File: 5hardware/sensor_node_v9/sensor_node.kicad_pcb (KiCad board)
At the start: 2 copper layers, 11.6 x 19.6 mm, 24 parts, among them J1 Conn_01x04_Pin, J3 Conn_01x04_Pin, Q1 BC818, Q2 Si2371EDS, Q3 AO3400A, U12 APDS-9960, U13 SHT31-DIS, U17 BH1750FVI-TR, U7 XC6206PxxxMR, U8 TPL5110

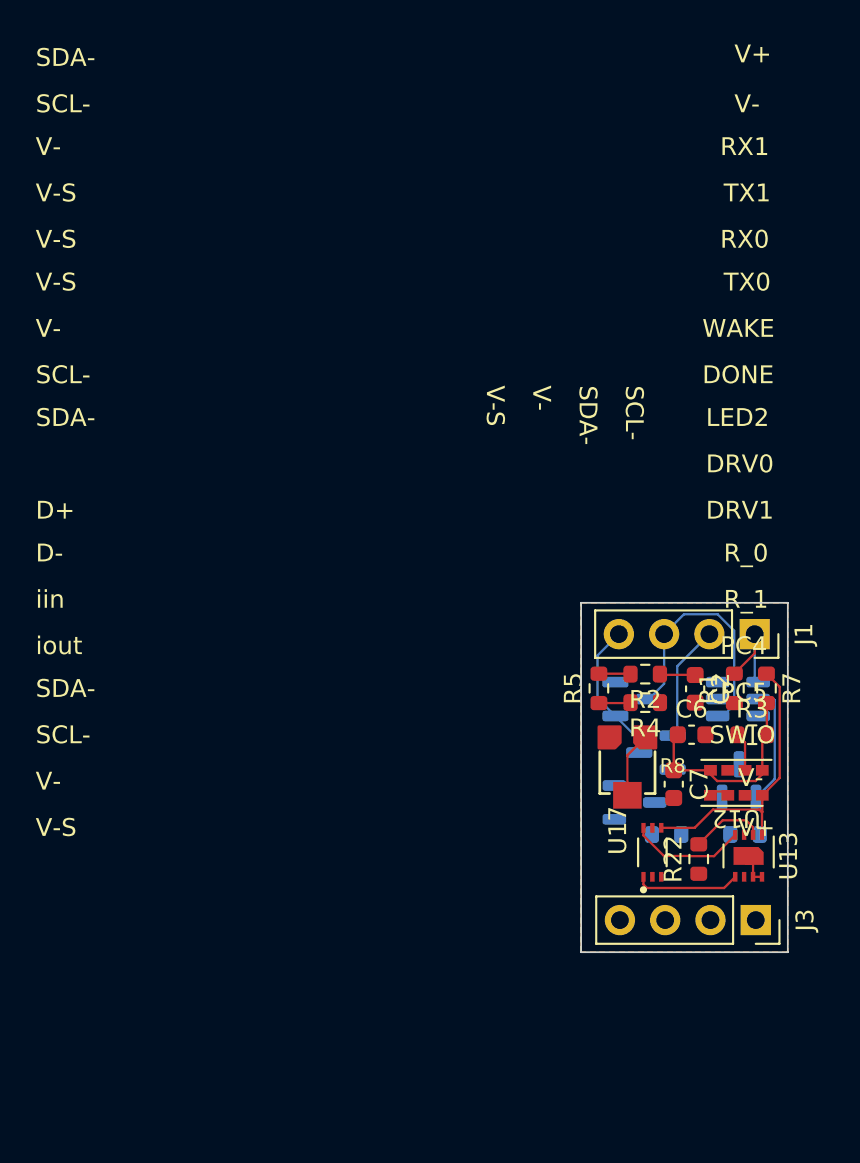
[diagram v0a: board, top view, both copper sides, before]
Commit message: update PCB.
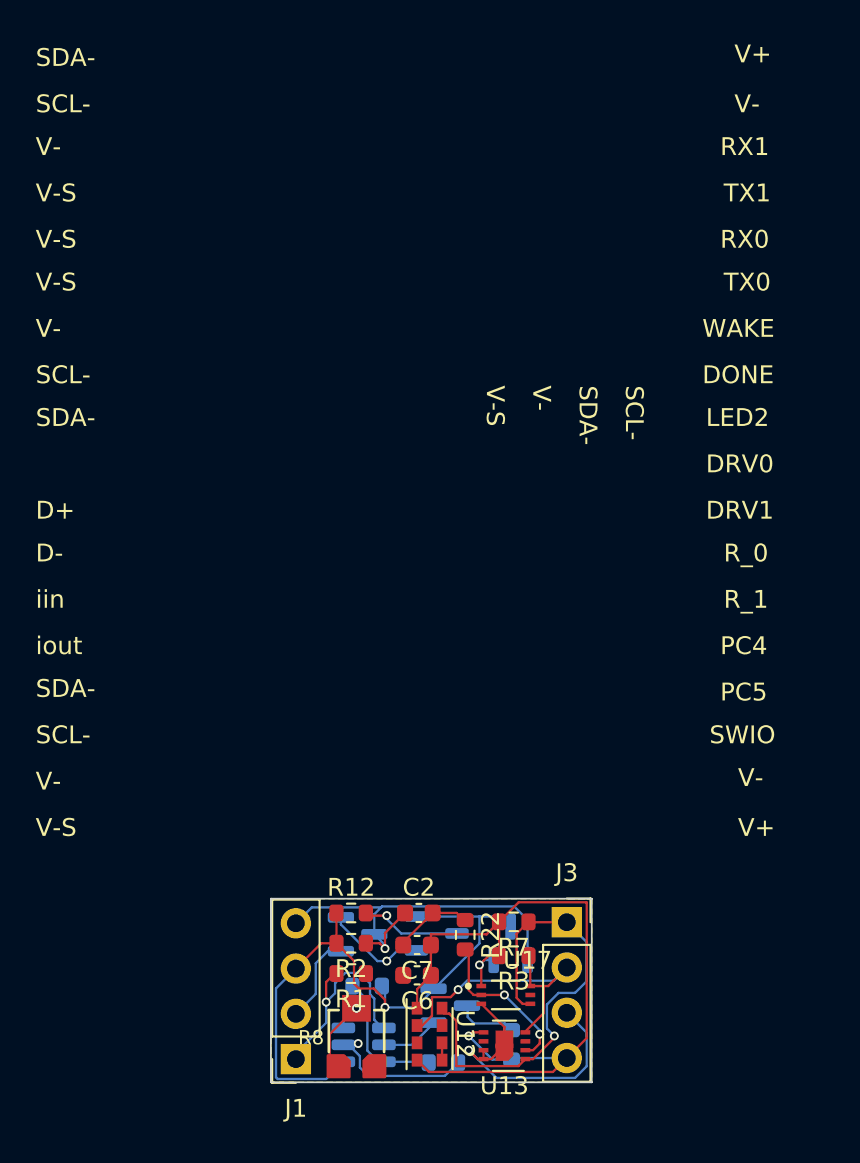
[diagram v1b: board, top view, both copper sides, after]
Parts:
- R12: moved to F.Cu
- R4, R5: moved to B.Cu
- moved J1 35.1 mm to (157.2, 98.2), turned to 180 degrees
- moved U8 28.6 mm to (161.0, 97.4)
- moved R1 26.8 mm to (160.3, 93.4), turned to 180 degrees
- moved R4 23.2 mm to (165.5, 98.4)
- moved R2 22.4 mm to (160.3, 91.7)
- moved U12 22.3 mm to (164.7, 96.8), turned to -90 degrees
- moved R8 21.5 mm to (160.6, 97.0), turned to 0 degrees
- moved R5 21.2 mm to (161.2, 94.1), turned to 0 degrees
- moved Q2 20.5 mm to (165.9, 95.2), turned to 0 degrees
- moved C6 20.5 mm to (164.0, 93.5), turned to 180 degrees
- moved C2 20.0 mm to (164.1, 90.0), turned to 0 degrees
- moved Q1 19.6 mm to (160.7, 91.2), turned to 0 degrees
- moved R7 19.3 mm to (169.4, 90.5), turned to 180 degrees
- moved R3 18.2 mm to (169.4, 92.4), turned to 180 degrees
- moved R12 18.2 mm to (160.3, 90.0), turned to 0 degrees
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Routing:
- net GND: track 1.78 -> 36.0 mm, vias 0 -> 3
- net +3.3V: track 17.7 -> 44.4 mm, vias 0 -> 2
- net GPIO: track 15.9 -> 35.2 mm, vias 0 -> 1
- net GPIO_GND: track 9.86 -> 23.1 mm, vias 0 -> 1
- net SDA-: track 15.9 -> 25.8 mm, vias 0 -> 1
- net SCL-: track 8.73 -> 17.6 mm, vias 0 -> 1
- net DONE: track 5.46 -> 12.4 mm, vias 0 -> 1
- net iout: track 0.00 -> 6.14 mm, vias 0 -> 1
- net Net-(U8-EN/ONE_SHOT): track 1.85 -> 7.72 mm
- net Net-(U13-ADDR): track 4.20 -> 8.76 mm, vias 0 -> 2
- net Net-(Q2-G): track 6.86 -> 3.34 mm
- net Net-(Q2-D): track 0.00 -> 3.41 mm
- net Net-(U8-DELAY/M_DRV): track 3.66 -> 5.51 mm, vias 0 -> 1
- net DRIVE: track 6.83 -> 4.99 mm
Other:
- board size 11.6 x 19.6 mm -> 18 x 10.3 mm
